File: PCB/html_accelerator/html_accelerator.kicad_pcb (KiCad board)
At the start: 4 copper layers, 129.3 x 104.4 mm, 170 parts, among them J1 Bus_PCI_Express_x16, J2 PCIexpress_bracket, U1 MCS9990, U10 AU6438BS, U11 EMMC_4G, U12 MCS9990, U2 AP1513, U3 CAT24C256YI-GT3, U4 AU6438BS, U5 EMMC_4G, U6 EMMC_4G, U7 EMMC_4G, U8 AU6438BS, U9 AU6438BS, Y1 12MHz, Y2 12MHz, Y3 12MHz, Y4 12MHz, Y5 12MHz

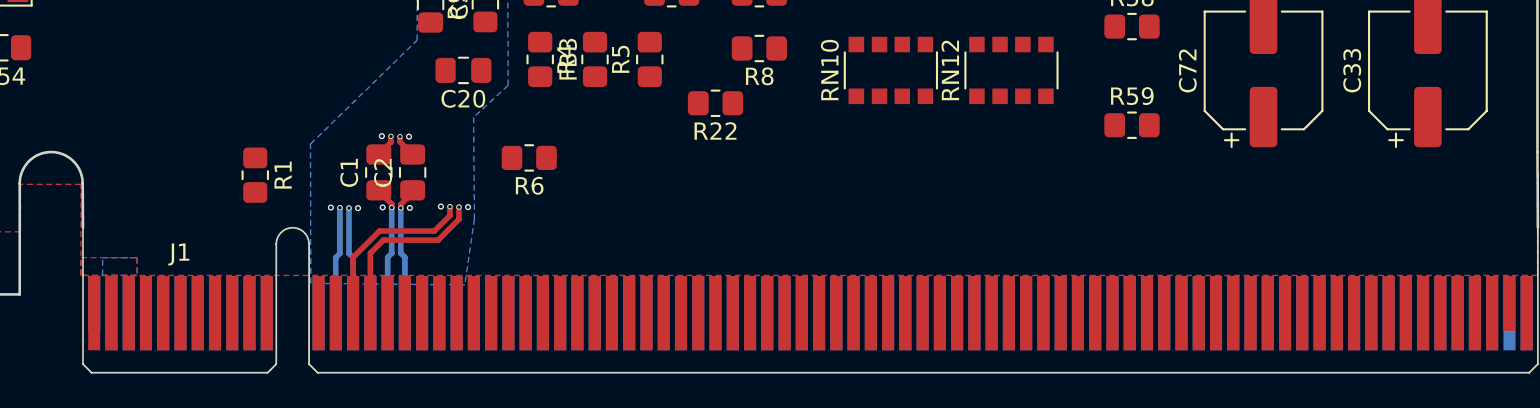
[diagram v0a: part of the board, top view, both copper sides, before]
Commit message: trace routing
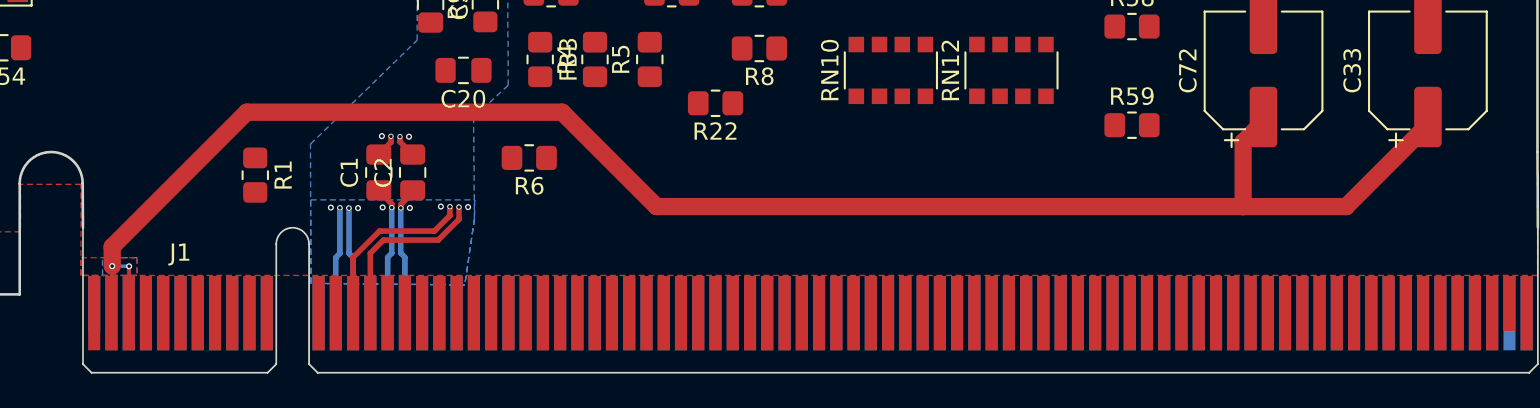
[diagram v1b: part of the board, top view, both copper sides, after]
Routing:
- net +12V: track 0.00 -> 101.1 mm, vias 0 -> 2
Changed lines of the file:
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@@
   )
   (target plus (at 159.467 159.533) (size 5) (width 0.05) (layer "Edge.Cuts"))
+  (segment (start 226.555 146.205) (end 227.755 145.005) (width 1) (layer "F.Cu") (net 4))
+  (segment (start 226.555 149.945) (end 226.555 146.205) (width 1) (layer "F.Cu") (net 4))
+  (segment (start 168.825 144.475) (end 187.095 144.475) (width 1) (layer "F.Cu") (net 4))
+  (segment (start 187.095 144.475) (end 192.565 149.945) (width 1) (layer "F.Cu") (net 4))
+  (segment (start 192.565 149.945) (end 226.555 149.945) (width 1) (layer "F.Cu") (net 4))
+  (segment (start 226.555 149.945) (end 232.525 149.945) (width 1) (layer "F.Cu") (net 4))
+  (segment (start 160.983 153.437) (end 161.025 153.395) (width 0.2) (layer "F.Cu") (net 4))
+  (segment (start 160.983 156.121) (end 160.983 153.437) (width 0.2) (layer "F.Cu") (net 4))
+  (segment (start 237.255 145.215) (end 237.255 144.925) (width 1) (layer "F.Cu") (net 4))
+  (segment (start 161.025 152.275) (end 161.025 152.145) (width 0.2) (layer "F.Cu") (net 4))
+  (segment (start 162.005 153.405) (end 162.005 156.115) (width 0.2) (layer "F.Cu") (net 4))
+  (segment (start 161.025 152.275) (end 168.825 144.475) (width 1) (layer "F.Cu") (net 4))
+  (segment (start 161.025 153.395) (end 161.025 152.275) (width 1) (layer "F.Cu") (net 4))
+  (segment (start 232.525 149.945) (end 237.255 145.215) (width 1) (layer "F.Cu") (net 4))
+  (via (at 161.025 153.395) (size 0.35) (drill 0.2) (layers "F.Cu" "B.Cu") (net 4))
+  (via (at 162.005 153.405) (size 0.35) (drill 0.2) (layers "F.Cu" "B.Cu") (net 4))
+  (segment (start 162.005 153.405) (end 162.005 155.475) (width 0.2) (layer "B.Cu") (net 4))
+  (segment (start 161.025 153.395) (end 161.995 153.395) (width 0.2) (layer "B.Cu") (net 4))
+  (segment (start 161.025 153.395) (end 161.025 155.305) (width 0.2) (layer "B.Cu") (net 4))
+  (segment (start 161.995 153.395) (end 162.005 153.405) (width 0.2) (layer "B.Cu") (net 4))
   (via (at 184.506401 130.015583) (size 0.35) (drill 0.2) (layers "F.Cu" "B.Cu") (free) (net 104))
   (via (at 176.651527 145.863238) (size 0.35) (drill 0.2) (layers "F.Cu" "B.Cu") (free) (net 104))
@@
       )
     )
+  )
+  (zone locked (net 104) (net_name "GND") (layer "B.Cu") (name "PCIE_SHIELD2") (hatch edge 0.5)
+    (priority 3)
+    (connect_pads (clearance 0))
+    (min_thickness 0.25) (filled_areas_thickness no)
+    (fill yes (thermal_gap 0.5) (thermal_bridge_width 0.5))
+    (polygon
+      (pts
+        (xy 181.455 154.485)
+        (xy 172.535 154.395)
+        (xy 172.525 149.555)
+        (xy 182.035 149.555)
+        (xy 182.015 150.655)
+      )
+    )
